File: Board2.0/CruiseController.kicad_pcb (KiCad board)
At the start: 2 copper layers, 23.1 x 38 mm, 56 parts, among them J1 USB_B_Micro, J2 Conn_02x09_Top_Bottom, U1 ADG884, U3 TLV9064IRTER, U5 MIC5225, U6 MCP2562-E-MF, U7 STM32L433CCUx, Y1 32.768

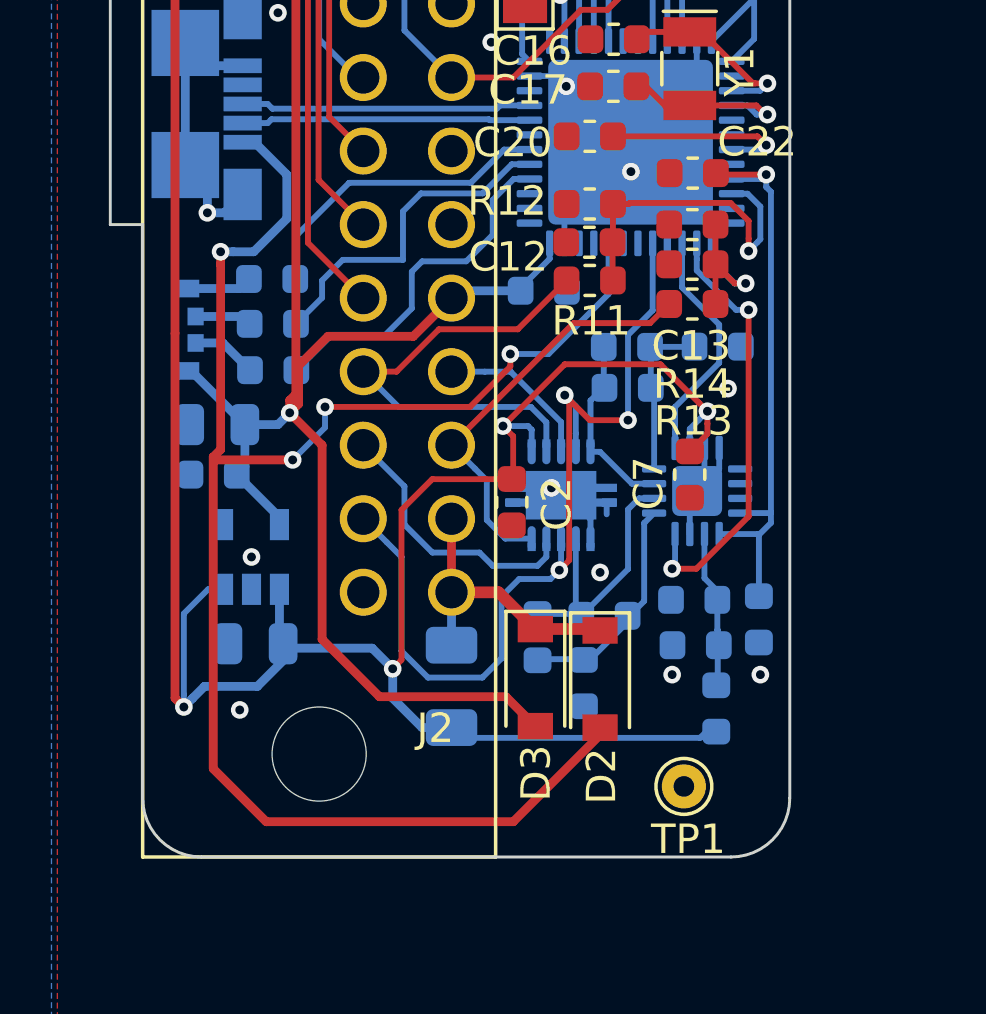
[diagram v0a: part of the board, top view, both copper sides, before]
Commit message: udpate v2 pcb
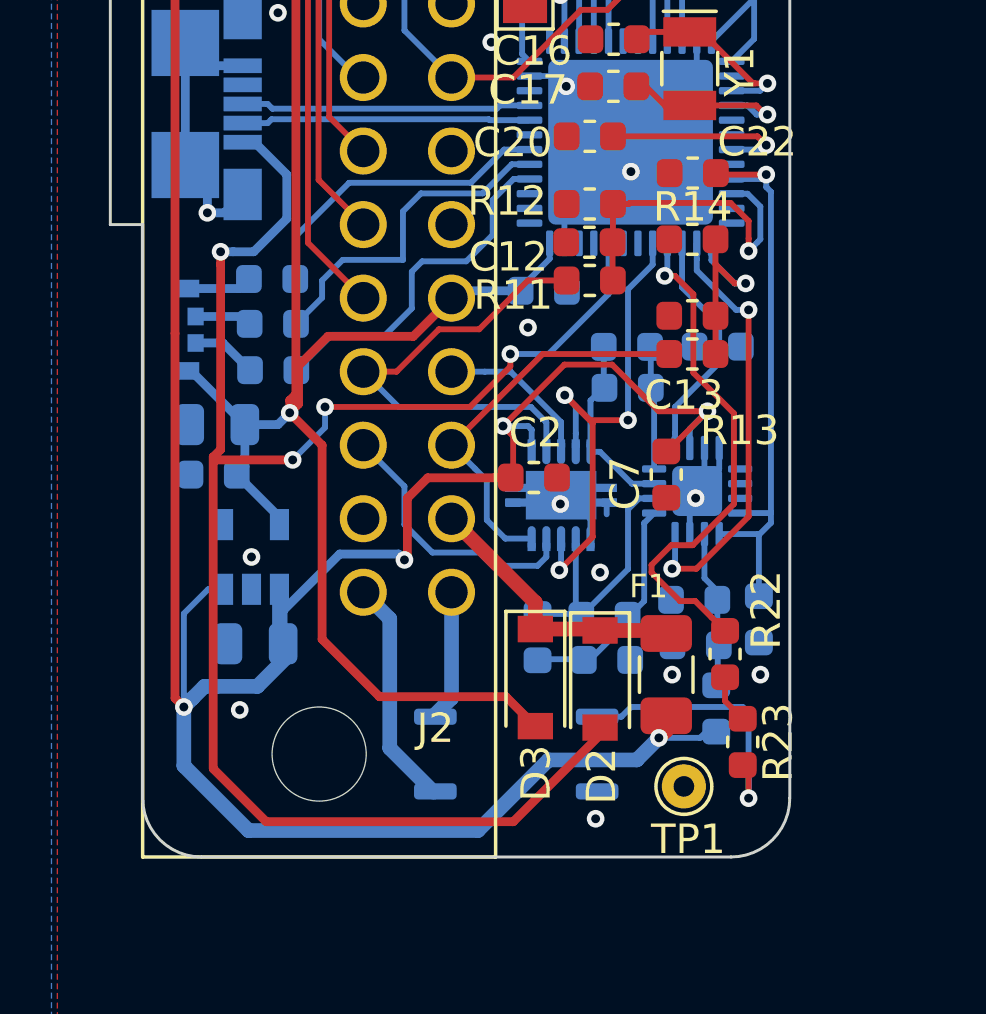
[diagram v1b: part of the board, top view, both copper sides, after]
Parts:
- added R22: 75, Resistor_SMD:R_0603_1608Metric, F.Cu at (119.8, 101.1)
- added R23: 75, Resistor_SMD:R_0603_1608Metric, F.Cu at (120.4, 104.1)
- added U2: CPC1017N, Package_SO:SOP-4_3.8x4.1mm_P2.54mm, B.Cu at (112.7, 104.5)
- F1: moved to F.Cu
- moved F1 7.31 mm to (117.8, 101.8)
- moved C13 3.10 mm to (118.7, 89.6)
- moved R13 1.70 mm to (118.7, 90.9)
- moved C2 1.12 mm to (113.3, 95.1), turned to 180 degrees
- moved R3 1.11 mm to (115.8, 101.3), turned to 180 degrees
- moved R14 0.85 mm to (118.7, 87.0)
- moved C7 0.80 mm to (117.8, 95.0)
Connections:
- J1 pad 4: Net-(J1-Pad4) -> (no net)
- J2 pad 1: VIN -> HZ1
- J2 pad 10: GND -> HZ0
- J2 pad 11: INTERSW -> GND
- U3 pad 5: Net-(U3-Pad5) -> (no net)
- U5 pad 4: Net-(U5-Pad4) -> (no net)
- U7 pad 11: Net-(U7-Pad11) -> (no net)
- U7 pad 12: Net-(U7-Pad12) -> (no net)
- U7 pad 16: Net-(U7-Pad16) -> HZEN
- U7 pad 18: Net-(U7-Pad18) -> (no net)
- U7 pad 19: Net-(U7-Pad19) -> (no net)
- U7 pad 2: Net-(U7-Pad2) -> (no net)
- U7 pad 21: Net-(U7-Pad21) -> (no net)
- U7 pad 22: Net-(U7-Pad22) -> (no net)
- U7 pad 25: Net-(U7-Pad25) -> (no net)
- U7 pad 26: Net-(U7-Pad26) -> (no net)
- U7 pad 27: Net-(U7-Pad27) -> (no net)
- U7 pad 31: Net-(U7-Pad31) -> (no net)
- U7 pad 34: Net-(U7-Pad34) -> (no net)
- U7 pad 37: Net-(U7-Pad37) -> (no net)
- U7 pad 42: Net-(U7-Pad42) -> (no net)
- U7 pad 43: Net-(U7-Pad43) -> (no net)
- U7 pad 5: Net-(U7-Pad5) -> (no net)
- U7 pad 6: Net-(U7-Pad6) -> (no net)
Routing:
- net HZEN: track 0.00 -> 17.3 mm, vias 0 -> 1
- net INTERSW: track 31.7 -> 18.9 mm
- net Net-(R23-Pad1): track 0.00 -> 9.48 mm, vias 0 -> 1
- net REGIN: track 106.5 -> 115.5 mm, vias 4 -> 5
- net HZ0: track 0.00 -> 7.79 mm
- net HZ1: track 0.00 -> 4.45 mm
- net Net-(R22-Pad1): track 0.00 -> 1.66 mm
- net VREFB: track 6.06 -> 6.96 mm
- net TTBIN: track 14.2 -> 13.5 mm
- net GND: vias 20 -> 22
